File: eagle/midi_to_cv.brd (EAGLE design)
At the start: 100 x 80 mm, 66 parts, among them IC1 4093N, Q3 2N3904, Q4 2N3904, Q5 2N3904, Q6 2SK30, U1 ATMEGA328P_PDIP

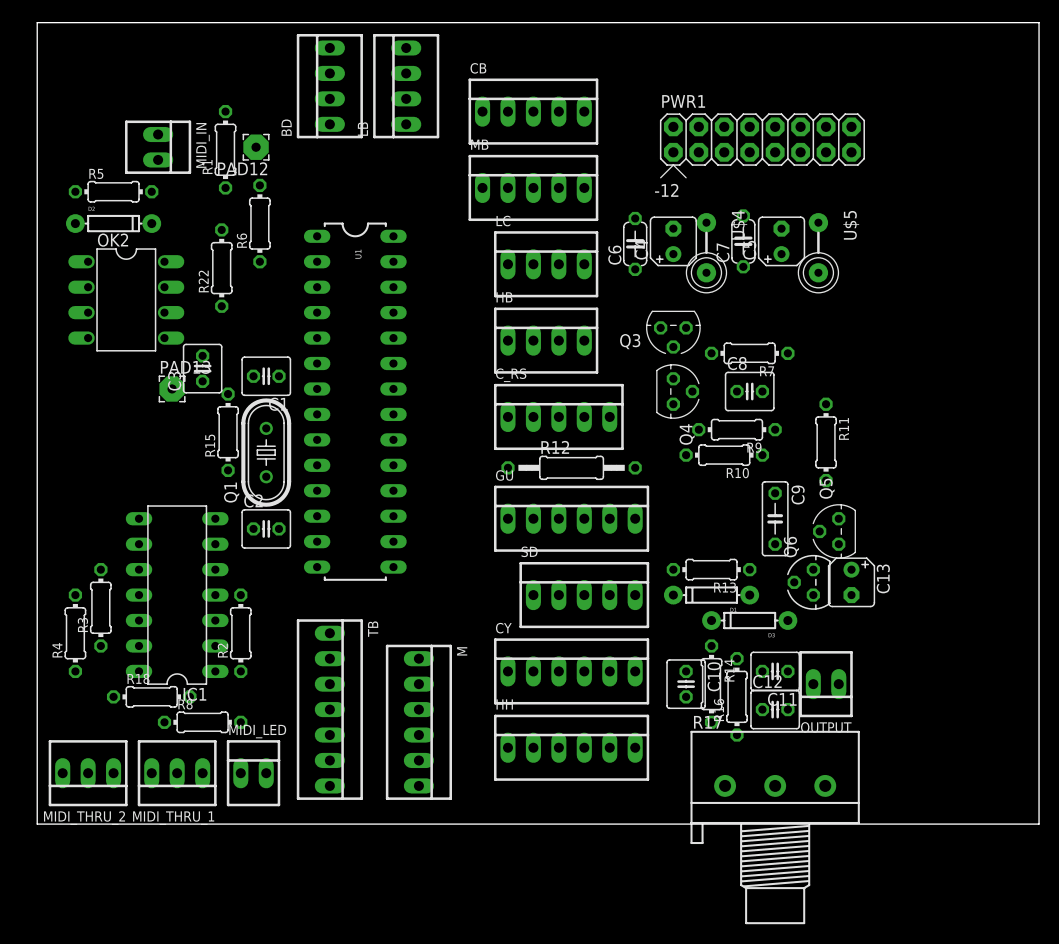
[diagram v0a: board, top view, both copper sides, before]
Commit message: 96pct auto
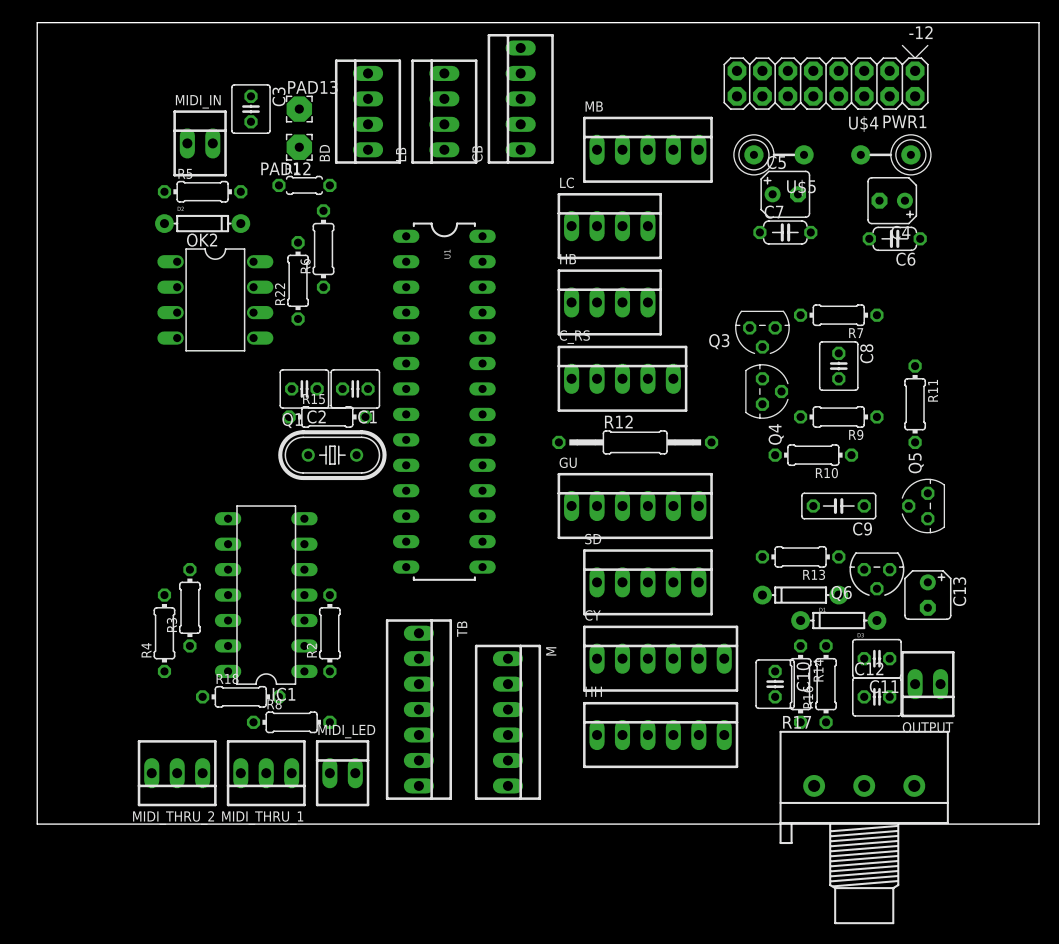
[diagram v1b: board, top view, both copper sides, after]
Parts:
- R1: device rcl:0204/7 -> rcl:0204/5
- R12: device rcl:0207/12 -> rcl:0207/15
- moved PAD13 30.7 mm to (26.2, 71.4)
- moved C3 26.4 mm to (21.3, 71.4), turned to 270 degrees
- moved C6 25.9 mm to (85.6, 58.4), turned to 180 degrees
- moved C4 22.2 mm to (85.3, 62.2), turned to 180 degrees
- moved U$4 20.2 mm to (84.7, 66.8), turned to 0 degrees
- moved C2 14.5 mm to (26.7, 43.4), turned to 180 degrees
- moved PWR1 12.7 mm to (81.3, 73.9), turned to 180 degrees
- moved MB 12.0 mm to (61.0, 67.3)
- moved R9 10.2 mm to (80.0, 40.6)
- moved C11 10.2 mm to (83.8, 16.5)
- moved C12 10.2 mm to (83.8, 12.7)
- moved OUTPUT 10.2 mm to (88.9, 14.0)
- moved U$5 10.1 mm to (74.0, 66.8), turned to 180 degrees
- moved R15 10.0 mm to (29.0, 40.6), turned to 0 degrees
- moved R11 9.67 mm to (87.6, 41.9)
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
